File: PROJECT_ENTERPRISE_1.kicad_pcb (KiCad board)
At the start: 4 copper layers, 90 x 40 mm, 63 parts, among them J1 USB_C_Receptacle_USB2.0_16P, J2 Battery Input, J3 Battery Input, J4 Battery Input, J5 Battery Input, Q2 IRF7343PBF, Q3 IRF7343PBF, Q4 IRF7343PBF, Q5 IRF7343PBF, U1 ESP32-S3-WROOM-1, U2 Nokia_5110_LCD, U3 LM2576T-3.3

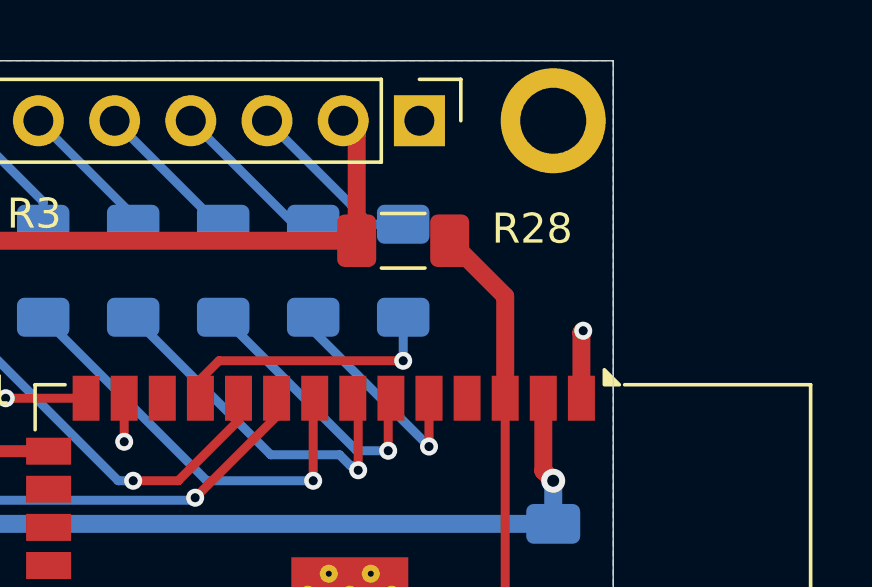
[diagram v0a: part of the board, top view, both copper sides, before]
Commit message: Added the rest
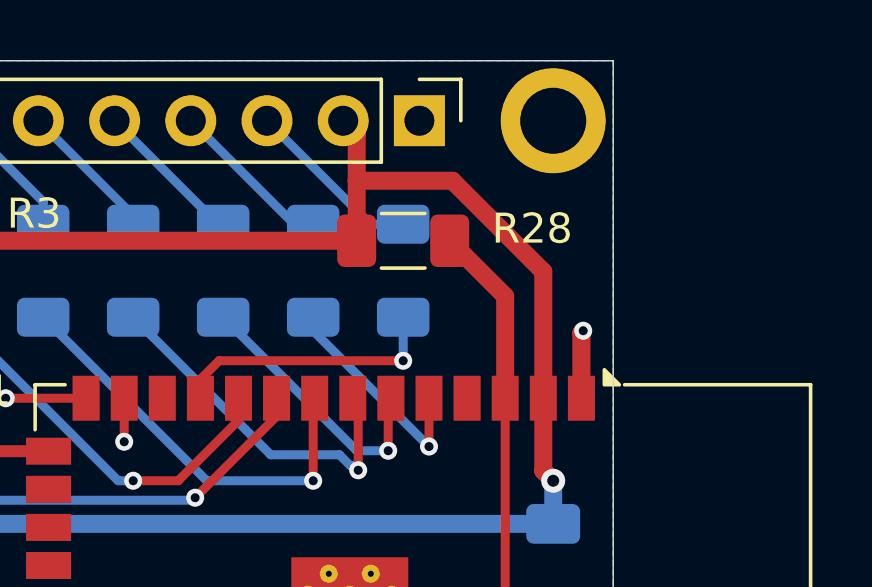
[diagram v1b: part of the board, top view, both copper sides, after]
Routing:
- net +3.3V: track 70.7 -> 82.4 mm
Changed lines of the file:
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@@
+	)
+	(segment
+		(start 232.622588 63.25)
+		(end 229.43 63.25)
+		(width 0.6)
+		(layer "F.Cu")
+		(net "+3.3V")
+	)
+	(segment
+		(start 235.65 66.277412)
+		(end 232.622588 63.25)
+		(width 0.6)
+		(layer "F.Cu")
+		(net "+3.3V")
+	)
+	(segment
+		(start 235.65 70.5)
+		(end 235.65 66.277412)
+		(width 0.6)
+		(layer "F.Cu")
+		(net "+3.3V")
+	)
+	(segment
+		(start 229.43 63.25)
+		(end 229.43 61.7)
+		(width 0.6)
+		(layer "F.Cu")
+		(net "+3.3V")
 	)
 	(segment
@@
 	(segment
 		(start 229.43 65.25)
-		(end 229.43 61.7)
+		(end 229.43 63.25)
 		(width 0.6)
 		(layer "F.Cu")

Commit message: Final product.
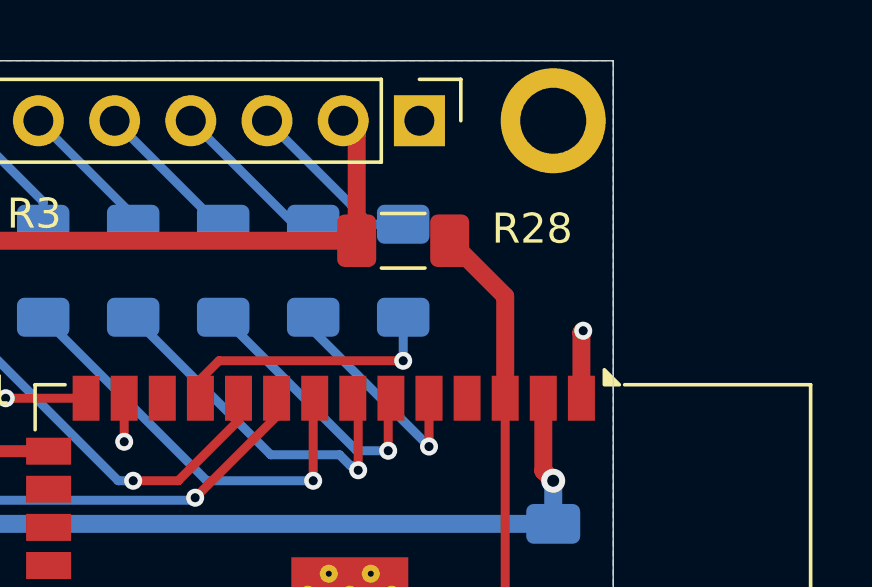
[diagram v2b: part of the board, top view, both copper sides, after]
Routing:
- net +3.3V: track 82.4 -> 70.7 mm
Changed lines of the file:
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@@
-	)
-	(segment
-		(start 232.622588 63.25)
-		(end 229.43 63.25)
-		(width 0.6)
-		(layer "F.Cu")
-		(net "+3.3V")
-	)
-	(segment
-		(start 235.65 66.277412)
-		(end 232.622588 63.25)
-		(width 0.6)
-		(layer "F.Cu")
-		(net "+3.3V")
-	)
-	(segment
-		(start 235.65 70.5)
-		(end 235.65 66.277412)
-		(width 0.6)
-		(layer "F.Cu")
-		(net "+3.3V")
-	)
-	(segment
-		(start 229.43 63.25)
-		(end 229.43 61.7)
-		(width 0.6)
-		(layer "F.Cu")
-		(net "+3.3V")
 	)
 	(segment
@@
 	(segment
 		(start 229.43 65.25)
-		(end 229.43 63.25)
+		(end 229.43 61.7)
 		(width 0.6)
 		(layer "F.Cu")
